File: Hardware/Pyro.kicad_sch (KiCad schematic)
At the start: 10 parts, among them J5 7788, J6 7788, Q4 BSZ025N04LS, U12 TCMT1109

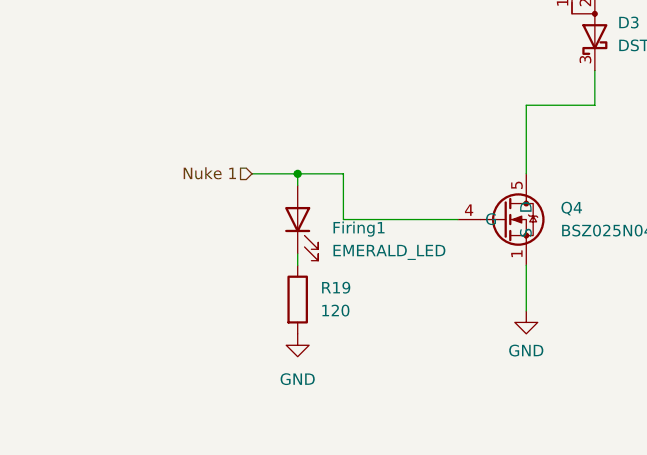
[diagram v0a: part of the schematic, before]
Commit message: Mega commit
Post review changes
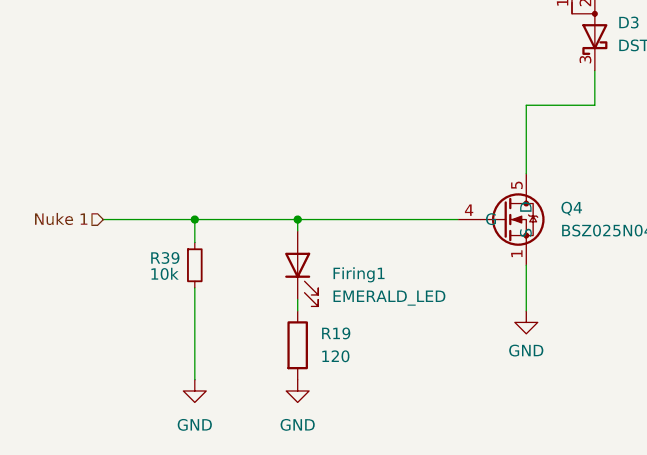
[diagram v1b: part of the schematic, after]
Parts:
- added R39: 10k, Resistor_SMD:R_0402_1005Metric, symbol Device:R_Small
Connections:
- net GND: now also R39.2
- net Nuke 1: now also R39.1
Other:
- moved on the sheet: Firing1, R19
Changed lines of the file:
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@@
+	)
+	(junction
+		(at 78.74 95.25)
+		(diameter 0)
+		(color 0 0 0 0)
 	)
 	(junction
@@
 	)
 	(junction
-		(at 90.17 90.17)
+		(at 90.17 95.25)
 		(diameter 0)
 		(color 0 0 0 0)
@@
 	(wire
 		(pts
-			(xy 90.17 99.06) (xy 90.17 100.33)
-		)
-		(stroke
-			(width 0)
-			(type default)
-		)
-	)
-	(wire
-		(pts
-			(xy 95.25 95.25) (xy 107.95 95.25)
+			(xy 78.74 95.25) (xy 90.17 95.25)
+		)
+		(stroke
+			(width 0)
+			(type default)
+		)
+	)
+	(wire
+		(pts
+			(xy 90.17 104.14) (xy 90.17 105.41)
 		)
 		(stroke
@@
 	(wire
 		(pts
-			(xy 95.25 90.17) (xy 95.25 95.25)
+			(xy 78.74 95.25) (xy 78.74 97.79)
 		)
 		(stroke
@@
 	(wire
 		(pts
-			(xy 85.09 90.17) (xy 90.17 90.17)
+			(xy 68.58 95.25) (xy 78.74 95.25)
 		)
 		(stroke
@@
 	(wire
 		(pts
-			(xy 90.17 90.17) (xy 95.25 90.17)
+			(xy 90.17 95.25) (xy 107.95 95.25)
+		)
+		(stroke
+			(width 0)
+			(type default)
+		)
+	)
+	(wire
+		(pts
+			(xy 78.74 102.87) (xy 78.74 113.03)
 		)
 		(stroke
@@
 	(wire
 		(pts
-			(xy 90.17 90.17) (xy 90.17 91.44)
+			(xy 90.17 95.25) (xy 90.17 96.52)
 		)
 		(stroke
@@
 	(hierarchical_label "Nuke 1"
 		(shape input)
-		(at 85.09 90.17 180)
+		(at 68.58 95.25 180)
 		(effects
 			(font
@@
 	)
 	(symbol
+		(lib_id "Device:R_Small")
+		(at 78.74 100.33 0)
+		(unit 1)
+		(exclude_from_sim no)
+		(in_bom yes)
+		(on_board yes)
+		(dnp no)
+		(property "Reference" "R39"
+			(at 75.438 99.568 0)
+			(effects
+				(font
+					(size 1.27 1.27)
+				)
+			)
+		)
+		(property "Value" "10k"
+			(at 75.3364 101.346 0)
+			(effects
+				(font
+					(size 1.27 1.27)
+				)
+			)
+		)
+		(property "Footprint" "Resistor_SMD:R_0402_1005Metric"
+			(at 78.74 100.33 0)
+			(effects
+				(font
+					(size 1.27 1.27)
+				)
+				(hide yes)
+			)
+		)
+		(property "Datasheet" "~"
+			(at 78.74 100.33 0)
+			(effects
+				(font
+					(size 1.27 1.27)
+				)
+				(hide yes)
+			)
+		)
+		(property "Description" ""
+			(at 78.74 100.33 0)
+			(effects
+				(font
+					(size 1.27 1.27)
+				)
+				(hide yes)
+			)
+		)
+		(pin "1"
+		)
+		(pin "2"
+		)
+		(instances
+			(project "Main board"
+				(path "/7db990e4-92e1-4f99-b4d2-435bbec1ba83/2f4d1188-68cf-4851-a56c-97d43238a03a"
+					(reference "R39")
+					(unit 1)
+				)
+			)
+		)
+	)
+	(symbol
 		(lib_id "power:GND")
-		(at 90.17 107.95 0)
+		(at 90.17 113.03 0)
 		(unit 1)
 		(exclude_from_sim no)
@@
 		(dnp no)
 		(property "Reference" "#PWR016"
-			(at 90.17 114.3 0)
+			(at 90.17 119.38 0)
 			(effects
 				(font
@@
 		)
 		(property "Value" "GND"
+			(at 90.17 118.11 0)
+			(effects
+				(font
+					(size 1.27 1.27)
+				)
+			)
+		)
+		(property "Footprint" ""
 			(at 90.17 113.03 0)
 			(effects
@@
 					(size 1.27 1.27)
 				)
-			)
-		)
-		(property "Footprint" ""
-			(at 90.17 107.95 0)
-			(effects
-				(font
-					(size 1.27 1.27)
-				)
 				(hide yes)
 			)
 		)
 		(property "Datasheet" ""
-			(at 90.17 107.95 0)
+			(at 90.17 113.03 0)
 			(effects
 				(font
@@
 		)
 		(property "Description" ""
-			(at 90.17 107.95 0)
+			(at 90.17 113.03 0)
 			(effects
 				(font
@@
 	)
 	(symbol
+		(lib_id "power:GND")
+		(at 78.74 113.03 0)
+		(unit 1)
+		(exclude_from_sim no)
+		(in_bom yes)
+		(on_board yes)
+		(dnp no)
+		(property "Reference" "#PWR073"
+			(at 78.74 119.38 0)
+			(effects
+				(font
+					(size 1.27 1.27)
+				)
+				(hide yes)
+			)
+		)
+		(property "Value" "GND"
+			(at 78.74 118.11 0)
+			(effects
+				(font
+					(size 1.27 1.27)
+				)
+			)
+		)
+		(property "Footprint" ""
+			(at 78.74 113.03 0)
+			(effects
+				(font
+					(size 1.27 1.27)
+				)
+				(hide yes)
+			)
+		)
+		(property "Datasheet" ""
+			(at 78.74 113.03 0)
+			(effects
+				(font
+					(size 1.27 1.27)
+				)
+				(hide yes)
+			)
+		)
+		(property "Description" ""
+			(at 78.74 113.03 0)
+			(effects
+				(font
+					(size 1.27 1.27)
+				)
+				(hide yes)
+			)
+		)
+		(pin "1"
+		)
+		(instances
+			(project "Main board"
+				(path "/7db990e4-92e1-4f99-b4d2-435bbec1ba83/2f4d1188-68cf-4851-a56c-97d43238a03a"
+					(reference "#PWR073")
+					(unit 1)
+				)
+			)
+		)
+	)
+	(symbol
 		(lib_id "Device:R")
-		(at 90.17 104.14 0)
+		(at 90.17 109.22 0)
 		(unit 1)
 		(exclude_from_sim no)
@@
 		(fields_autoplaced yes)
 		(property "Reference" "R19"
-			(at 92.71 102.8699 0)
+			(at 92.71 107.9499 0)
 			(effects
 				(font
@@
 		)
 		(property "Value" "120"
-			(at 92.71 105.4099 0)
+			(at 92.71 110.4899 0)
 			(effects
 				(font
@@
 		)
 		(property "Footprint" "Resistor_SMD:R_0402_1005Metric"
-			(at 88.392 104.14 90)
+			(at 88.392 109.22 90)
 			(effects
 				(font
@@
 		)
 		(property "Datasheet" "~"
-			(at 90.17 104.14 0)
+			(at 90.17 109.22 0)
 			(effects
 				(font
@@
 		)
 		(property "Description" ""
-			(at 90.17 104.14 0)
+			(at 90.17 109.22 0)
 			(effects
 				(font
@@
 	(symbol
 		(lib_id "Device:LED")
-		(at 90.17 95.25 90)
+		(at 90.17 100.33 90)
 		(unit 1)
 		(exclude_from_sim no)
@@
 		(fields_autoplaced yes)
 		(property "Reference" "Firing1"
-			(at 93.98 96.2025 90)
+			(at 93.98 101.2825 90)
 			(effects
 				(font
@@
 		)
 		(property "Value" "EMERALD_LED"
-			(at 93.98 98.7425 90)
+			(at 93.98 103.8225 90)
 			(effects
 				(font
@@
 		)
 		(property "Footprint" "LED_SMD:LED_0402_1005Metric"
-			(at 90.17 95.25 0)
+			(at 90.17 100.33 0)
 			(effects
 				(font
@@
 		)
 		(property "Datasheet" "~"
-			(at 90.17 95.25 0)
+			(at 90.17 100.33 0)
 			(effects
 				(font
@@
 		)
 		(property "Description" ""
-			(at 90.17 95.25 0)
-			(effects
-				(font
+			(at 90.17 100.33 0)
+			(effects
+				(font
